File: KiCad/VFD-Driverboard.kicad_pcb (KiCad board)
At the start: 2 copper layers, 100 x 25 mm, 2 parts, among them J2 Breadboard

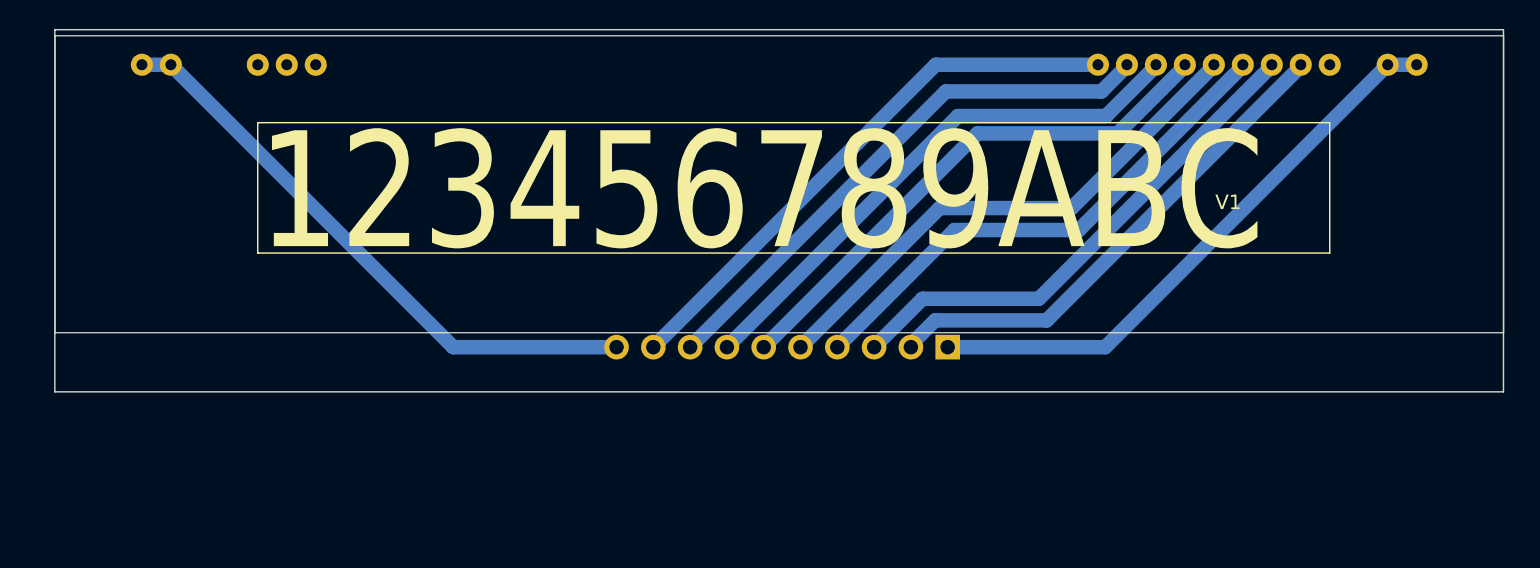
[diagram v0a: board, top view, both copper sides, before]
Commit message: new PCB
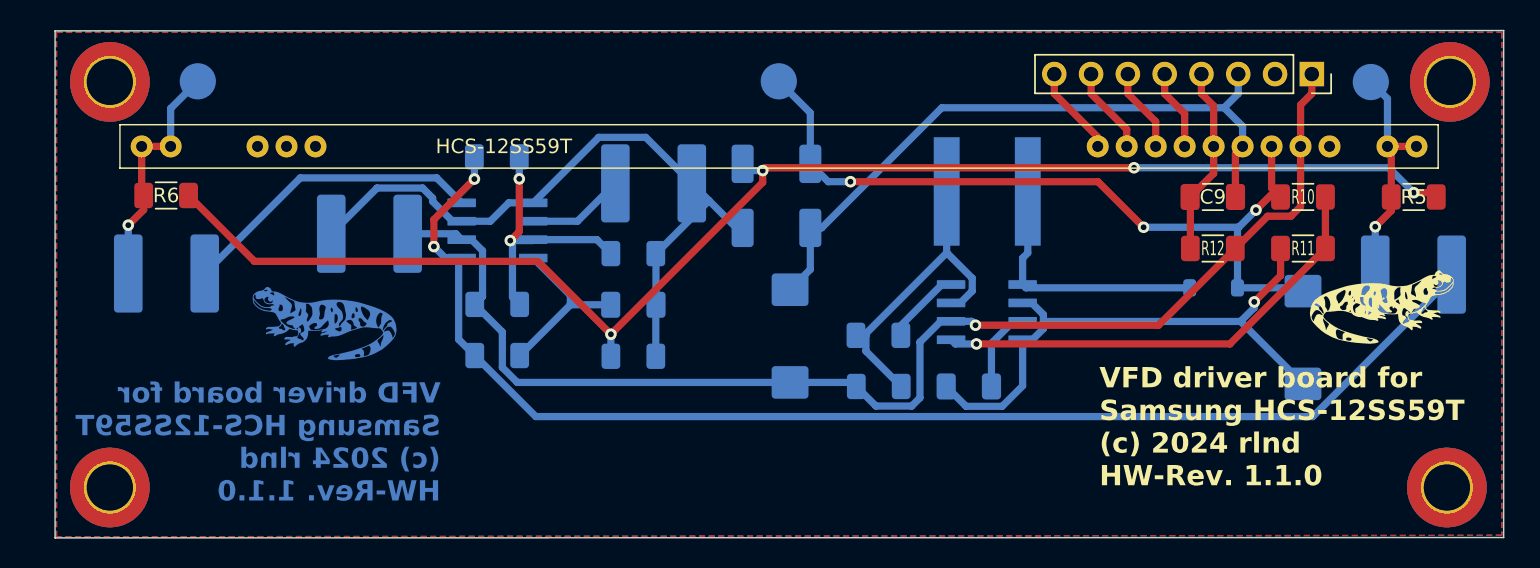
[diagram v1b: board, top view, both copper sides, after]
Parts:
- removed J2: Breadboard, Connector_PinHeader_2.54mm:PinHeader_1x10_P2.54mm_Vertical
- added C1: 1u, Capacitor_SMD:C_2220_5750Metric_Pad1.97x5.40mm_HandSolder, B.Cu at (35.1, 27.5)
- added C2: 10n, Capacitor_SMD:C_1206_3216Metric_Pad1.33x1.80mm_HandSolder, B.Cu at (53.3, 32.4)
- added C3: 1u, Capacitor_SMD:C_2220_5750Metric_Pad1.97x5.40mm_HandSolder, B.Cu at (107.2, 30.3)
- added C4: 1u, Capacitor_SMD:C_2220_5750Metric_Pad1.97x5.40mm_HandSolder, B.Cu at (21.1, 30.2)
- added C5: 1u, Capacitor_SMD:C_2220_5750Metric_Pad1.97x5.40mm_HandSolder, B.Cu at (54.7, 24.0)
- added C6: 100uF, Capacitor_Tantalum_SMD:CP_EIA-7343-31_Kemet-D_Pad2.25x2.55mm_HandSolder, B.Cu at (64.2, 34.5)
- added C7: 270pF, Capacitor_SMD:C_1206_3216Metric_Pad1.33x1.80mm_HandSolder, B.Cu at (76.5, 38.0)
- added C8: 100uF, Capacitor_Tantalum_SMD:CP_EIA-7343-31_Kemet-D_Pad2.25x2.55mm_HandSolder, B.Cu at (99.6, 34.6)
- added C9: 82p, Capacitor_SMD:C_1206_3216Metric_Pad1.33x1.80mm_HandSolder, F.Cu at (93.3, 24.9)
- added D1: 2V7, Diode_SMD:D_2010_5025Metric_Pad1.52x2.65mm_HandSolder, B.Cu at (63.2, 22.6)
- added D2: 1N5819, Diode_SMD:D_SOD-123, B.Cu at (93.4, 31.2)
- added D3: D, Diode_SMD:D_2010_5025Metric_Pad1.52x2.65mm_HandSolder, B.Cu at (63.2, 27.1)
- added G***: LOGO, MyLib:Salamander_Silk, F.Cu at (105.0, 32.5)
- added G***: LOGO, MyLib:Salamander_B_Copper, F.Cu at (32.0, 33.6)
- added H1: MountingHole, MountingHole:MountingHole_3.2mm_M3_ISO14580_Pad_TopBottom, F.Cu at (17.2, 17.0)
- added H2: MountingHole, MountingHole:MountingHole_3.2mm_M3_ISO14580_Pad_TopBottom, F.Cu at (109.7, 17.0)
- added H3: MountingHole, MountingHole:MountingHole_3.2mm_M3_ISO14580_Pad_TopBottom, F.Cu at (17.2, 45.0)
- added H4: MountingHole, MountingHole:MountingHole_3.2mm_M3_ISO14580_Pad_TopBottom, F.Cu at (109.5, 45.0)
- added J1: MCU, Connector_PinSocket_2.54mm:PinSocket_1x08_P2.54mm_Vertical, F.Cu at (100.2, 16.4)
- added L1: 100uH, MyLib:IND_TAIYO_NRS8040_TAY, B.Cu at (77.8, 24.5)
- added R1: 10k, Resistor_SMD:R_1206_3216Metric_Pad1.30x1.75mm_HandSolder, B.Cu at (43.9, 32.3)
- added R10: 47k, Resistor_SMD:R_1206_3216Metric_Pad1.30x1.75mm_HandSolder, F.Cu at (99.6, 24.9)
- added R11: 1k8, Resistor_SMD:R_1206_3216Metric_Pad1.30x1.75mm_HandSolder, F.Cu at (99.6, 28.5)
- added R12: 8k2, Resistor_SMD:R_1206_3216Metric_Pad1.30x1.75mm_HandSolder, F.Cu at (93.3, 28.5)
- added R2: 10k, Resistor_SMD:R_1206_3216Metric_Pad1.30x1.75mm_HandSolder, B.Cu at (53.3, 28.8)
- added R3: 2k2, Resistor_SMD:R_1206_3216Metric_Pad1.30x1.75mm_HandSolder, B.Cu at (43.9, 35.9)
- added R4: 10k, Resistor_SMD:R_1206_3216Metric_Pad1.30x1.75mm_HandSolder, B.Cu at (43.9, 22.2)
- added R5: 1k, Resistor_SMD:R_1206_3216Metric_Pad1.30x1.75mm_HandSolder, F.Cu at (107.2, 24.9)
- added R6: 1k, Resistor_SMD:R_1206_3216Metric_Pad1.30x1.75mm_HandSolder, F.Cu at (21.1, 24.8)
- added R7: 100k, Resistor_SMD:R_1206_3216Metric_Pad1.30x1.75mm_HandSolder, B.Cu at (53.3, 35.9)
- added R8: 1, Resistor_SMD:R_1206_3216Metric_Pad1.30x1.75mm_HandSolder, B.Cu at (70.3, 38.0)
- added R9: 180, Resistor_SMD:R_1206_3216Metric_Pad1.30x1.75mm_HandSolder, B.Cu at (70.2, 34.5)
- added TP1: VEE, TestPoint:TestPoint_Pad_D2.5mm, B.Cu at (63.4, 16.9)
- added TP2: F-, TestPoint:TestPoint_Pad_D2.5mm, B.Cu at (104.2, 17.0)
- added TP3: F+, TestPoint:TestPoint_Pad_D2.5mm, B.Cu at (23.3, 16.9)
- added U1: MC34063, MyLib:SOIC127P599X175-8N, B.Cu at (77.7, 32.9)
- added U2: LM4871, MyLib:SOIC127P599X175-8N, B.Cu at (44.0, 27.2)
- V1: value ~ -> HCS-12SS59T
- moved V1 5.44 mm to (13.4, 19.4)
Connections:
- V1 pad 7: GNDD -> Gnd
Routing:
- net Net-(D1-K): track 0.00 -> 99.3 mm, vias 0 -> 4
- net Net-(U2-V01): track 0.00 -> 90.2 mm, vias 0 -> 2
- net VCC: track 35.2 -> 88.6 mm, vias 0 -> 1
- net Net-(D3-K): track 0.00 -> 48.1 mm
- net Gnd: track 0.00 -> 46.5 mm
- net Net-(U1-GND): track 0.00 -> 40.0 mm, vias 0 -> 1
- net GNDD: track 36.1 -> 0.00 mm
- net Net-(J1-Pin_8): track 38.8 -> 6.24 mm
- net Net-(J1-Pin_7): track 38.3 -> 6.01 mm
- net Net-(U1-Vfb): track 0.00 -> 32.3 mm, vias 0 -> 1
- net Net-(J1-Pin_6): track 37.7 -> 5.79 mm
- net Net-(J1-Pin_5): track 37.2 -> 5.57 mm
- net VF2: track 40.8 -> 16.5 mm, vias 0 -> 1
- net VF1: track 40.4 -> 16.2 mm, vias 0 -> 1
- net Net-(J1-Pin_4): track 36.7 -> 13.1 mm
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- added copper zone on B.Cu, net Gnd
- added copper zone on F.Cu, net Gnd
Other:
- board size 100 x 25 mm -> 100 x 35 mm
- board text added: "VFD driver board for Samsung HCS-12SS59T (c) 2024 rlnd HW-Rev. 1.1.0"
